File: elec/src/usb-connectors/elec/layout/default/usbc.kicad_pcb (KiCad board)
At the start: 2 copper layers, 3 parts

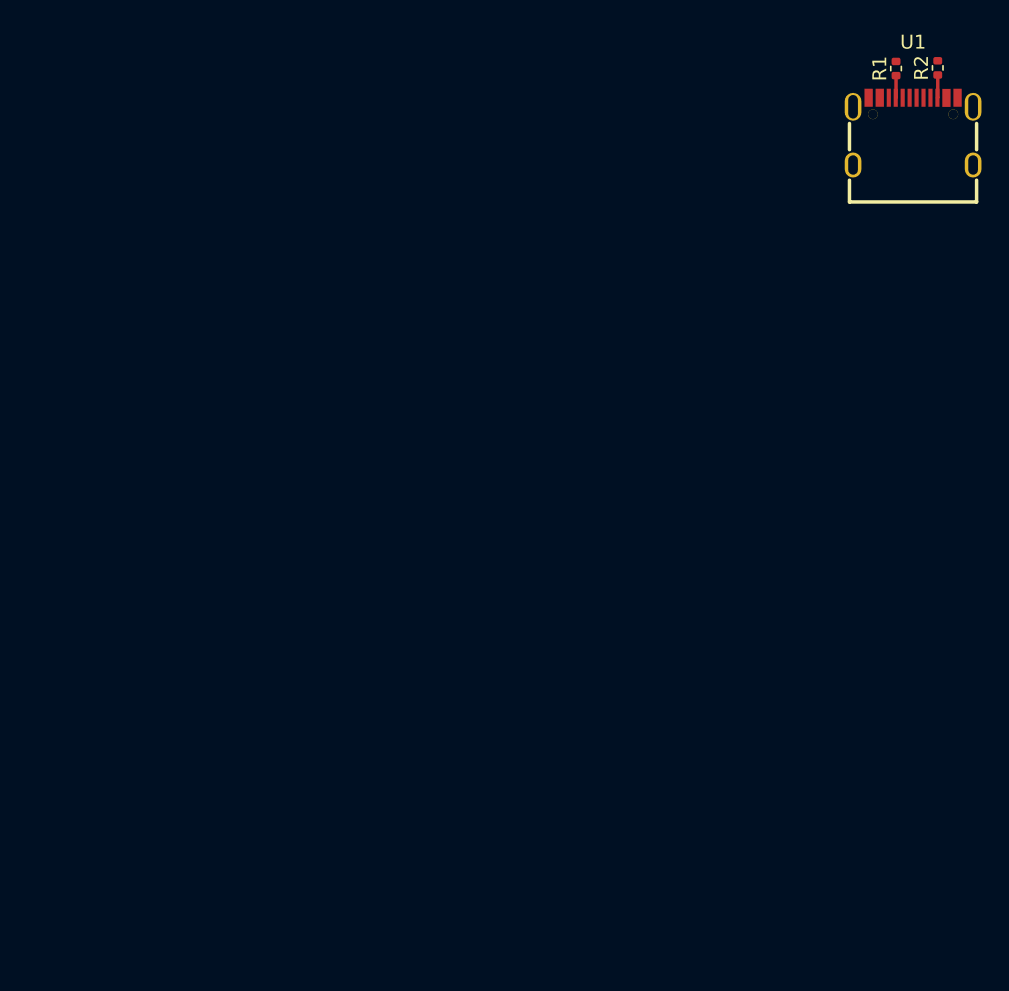
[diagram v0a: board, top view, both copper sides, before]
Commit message: working!!!
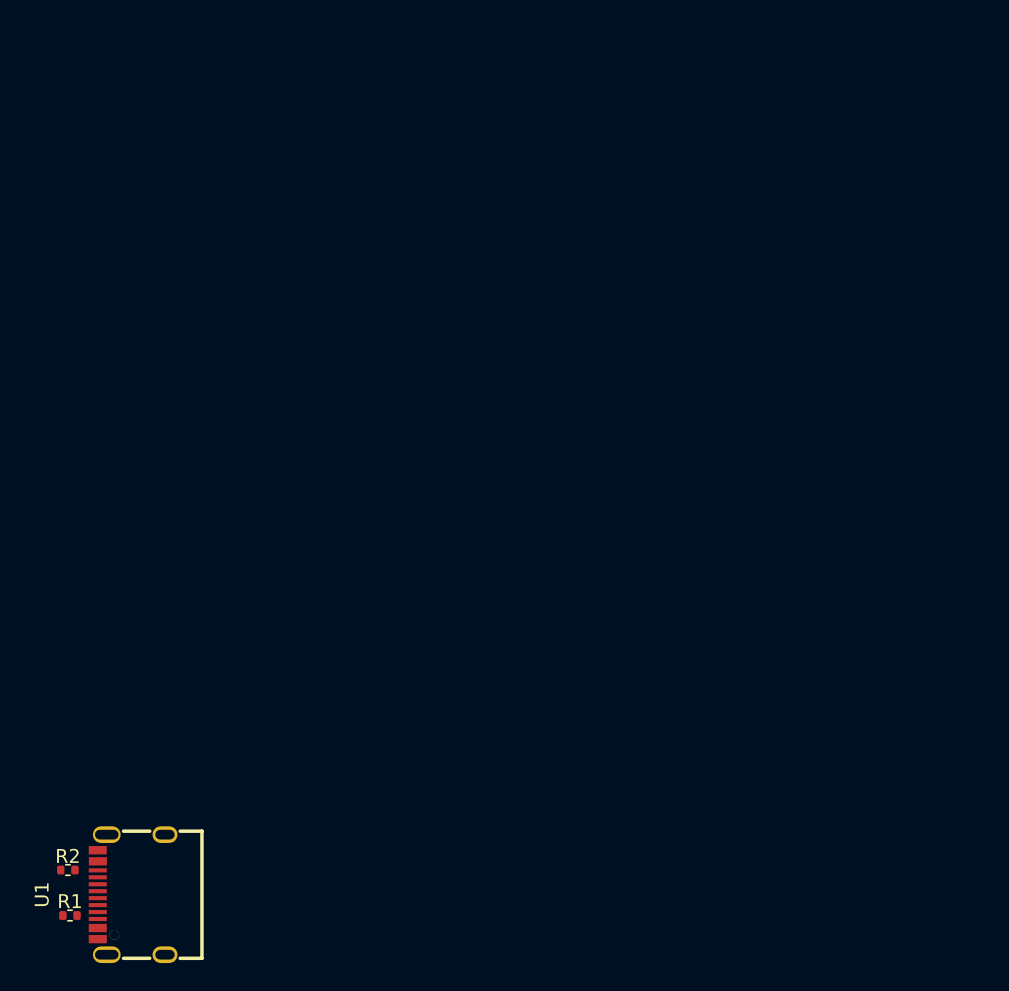
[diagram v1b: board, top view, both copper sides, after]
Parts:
- moved R2 85.2 mm to (69.8, 118.1), turned to 180 degrees
- moved R1 85.1 mm to (69.9, 121.4), turned to 180 degrees
- moved U1 78.6 mm to (74.4, 119.9), turned to 90 degrees
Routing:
- net cc2: track 1.65 -> 0.00 mm
- net cc1: track 1.60 -> 0.03 mm
